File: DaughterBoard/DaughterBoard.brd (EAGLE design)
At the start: 27.6 x 20.9 mm, 6 parts

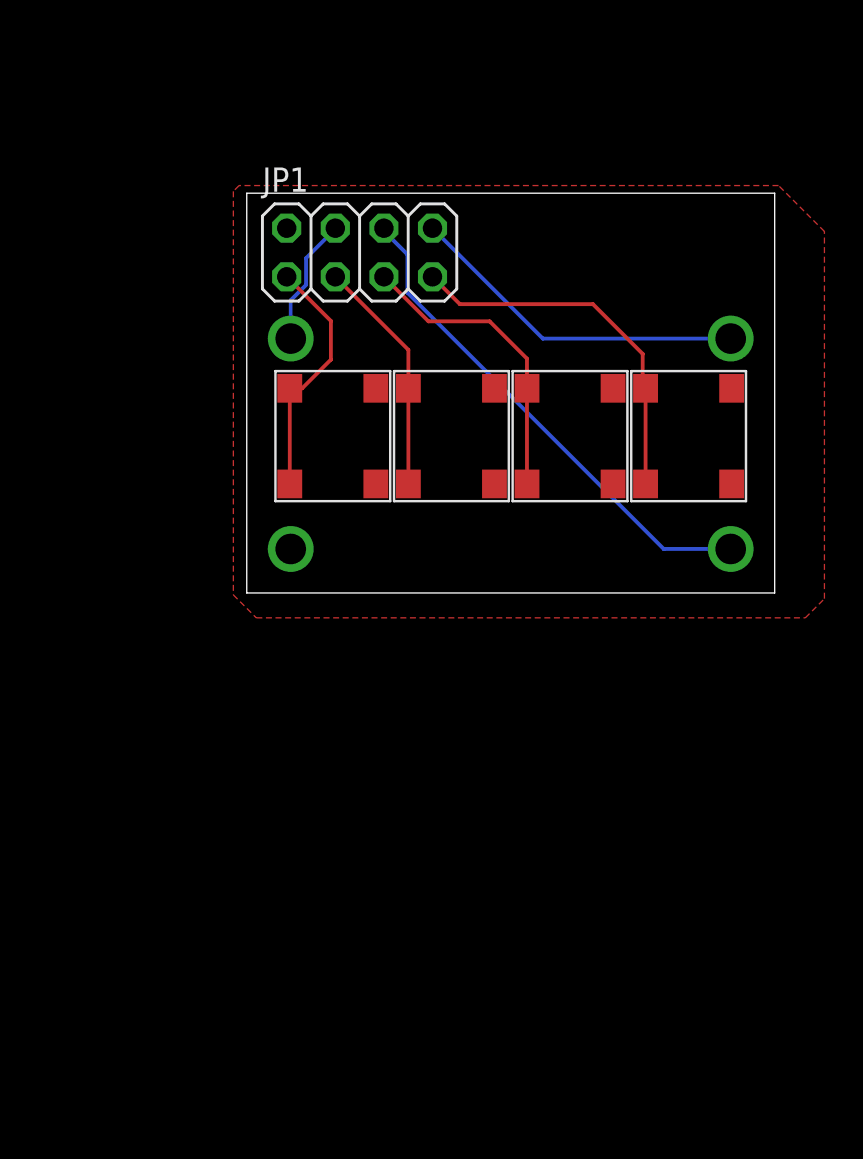
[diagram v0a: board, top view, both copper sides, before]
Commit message: Finished modified daughterboard
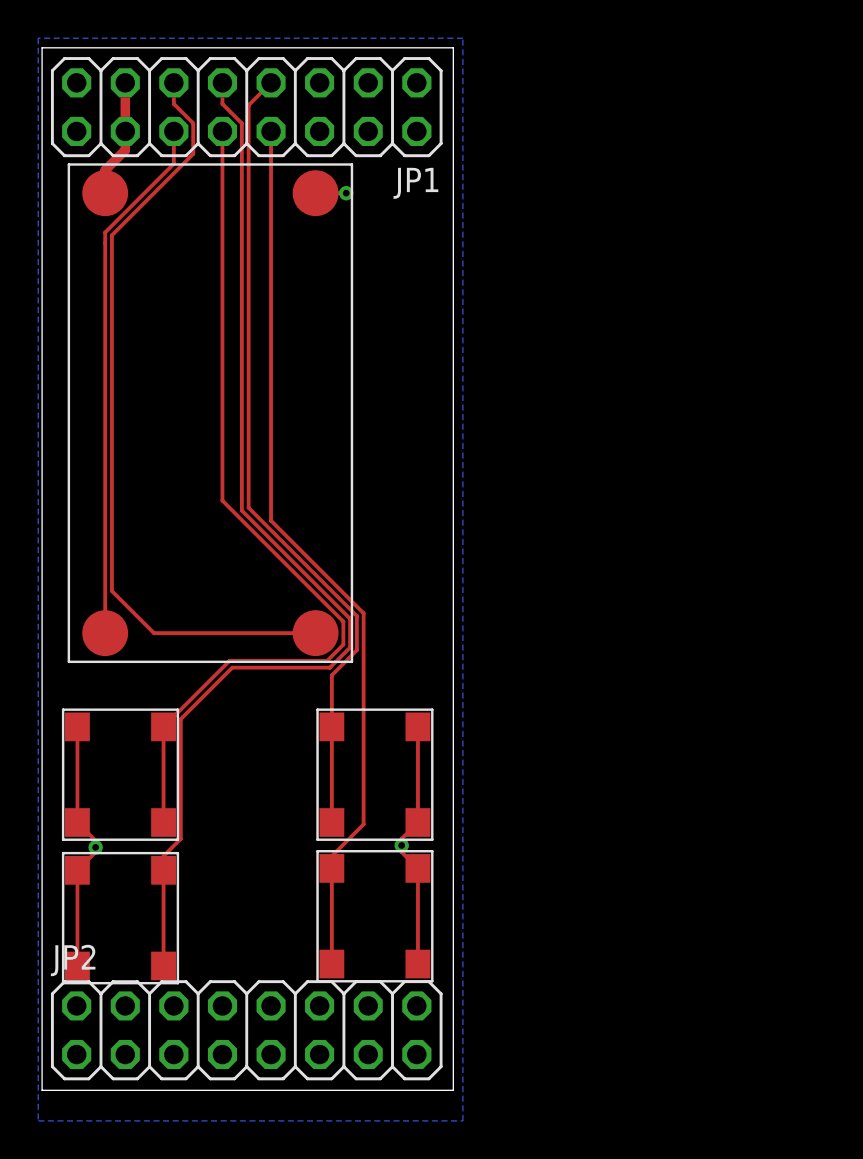
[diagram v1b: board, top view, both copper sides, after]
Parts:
- added JP2: (no value), pinhead:2X08
- JP1: device pinhead:2X04 -> pinhead:2X08
- moved U$5 34.6 mm to (-6.60, -9.50), turned to 90 degrees
- moved U$3 30.6 mm to (-6.60, -17.0), turned to 90 degrees
- moved U$4 27.1 mm to (6.70, -16.9)
- moved U$2 17.8 mm to (6.70, -9.50)
- moved U$1 15.8 mm to (-1.90, 9.40), flipped to the top, turned to 0 degrees
- moved JP1 9.62 mm to (0.00, 25.4), turned to 180 degrees
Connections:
- net +5V: now also JP1.13, JP1.14; no longer JP1.4
- net GND: now also JP1.15, JP1.16; no longer JP1.2
- net MUTP: now also JP1.10, U$5.3, U$5.4; no longer JP1.5, U$4.3, U$4.4
- net MUTR: now also JP1.9, U$3.3, U$3.4; no longer JP1.1, U$2.3, U$2.4
- net POE+: now also JP1.12; no longer JP1.8
- net POE-: now also JP1.11; no longer JP1.6
- net VLDN: now also JP1.7, U$2.3, U$2.4; no longer JP1.3, U$3.3, U$3.4
- net VLUP: now also JP1.8, U$4.3, U$4.4; no longer JP1.7, U$5.3, U$5.4
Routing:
- net MUTR: track 13.1 -> 56.0 mm
- net MUTP: track 15.8 -> 45.6 mm
- net VLDN: track 12.4 -> 42.0 mm
- net GND: track 0.00 -> 28.0 mm, vias 0 -> 3
- net VLUP: track 19.5 -> 46.2 mm
- net POE-: track 26.3 -> 40.3 mm
- net POE+: track 18.0 -> 27.7 mm
- net +5V: track 6.74 -> 6.20 mm
- added copper zone on layer 16, net GND
- removed copper zone on layer 1, net GND
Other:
- board size 27.6 x 20.9 mm -> 21.5 x 54.5 mm
